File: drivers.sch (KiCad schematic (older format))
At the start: 40 parts, among them J10 Conn_01x04_Male, J11 Conn_01x04_Male, J12 Conn_01x02_Male, J13 Conn_01x02_Male, J14 Conn_01x02_Male, J15 Conn_01x02_Male, J4 Conn_01x04_Male, J5 Conn_01x04_Male, J6 Conn_01x02_Male, J7 Conn_01x02_Male, J8 Conn_01x02_Male, J9 Conn_01x02_Male

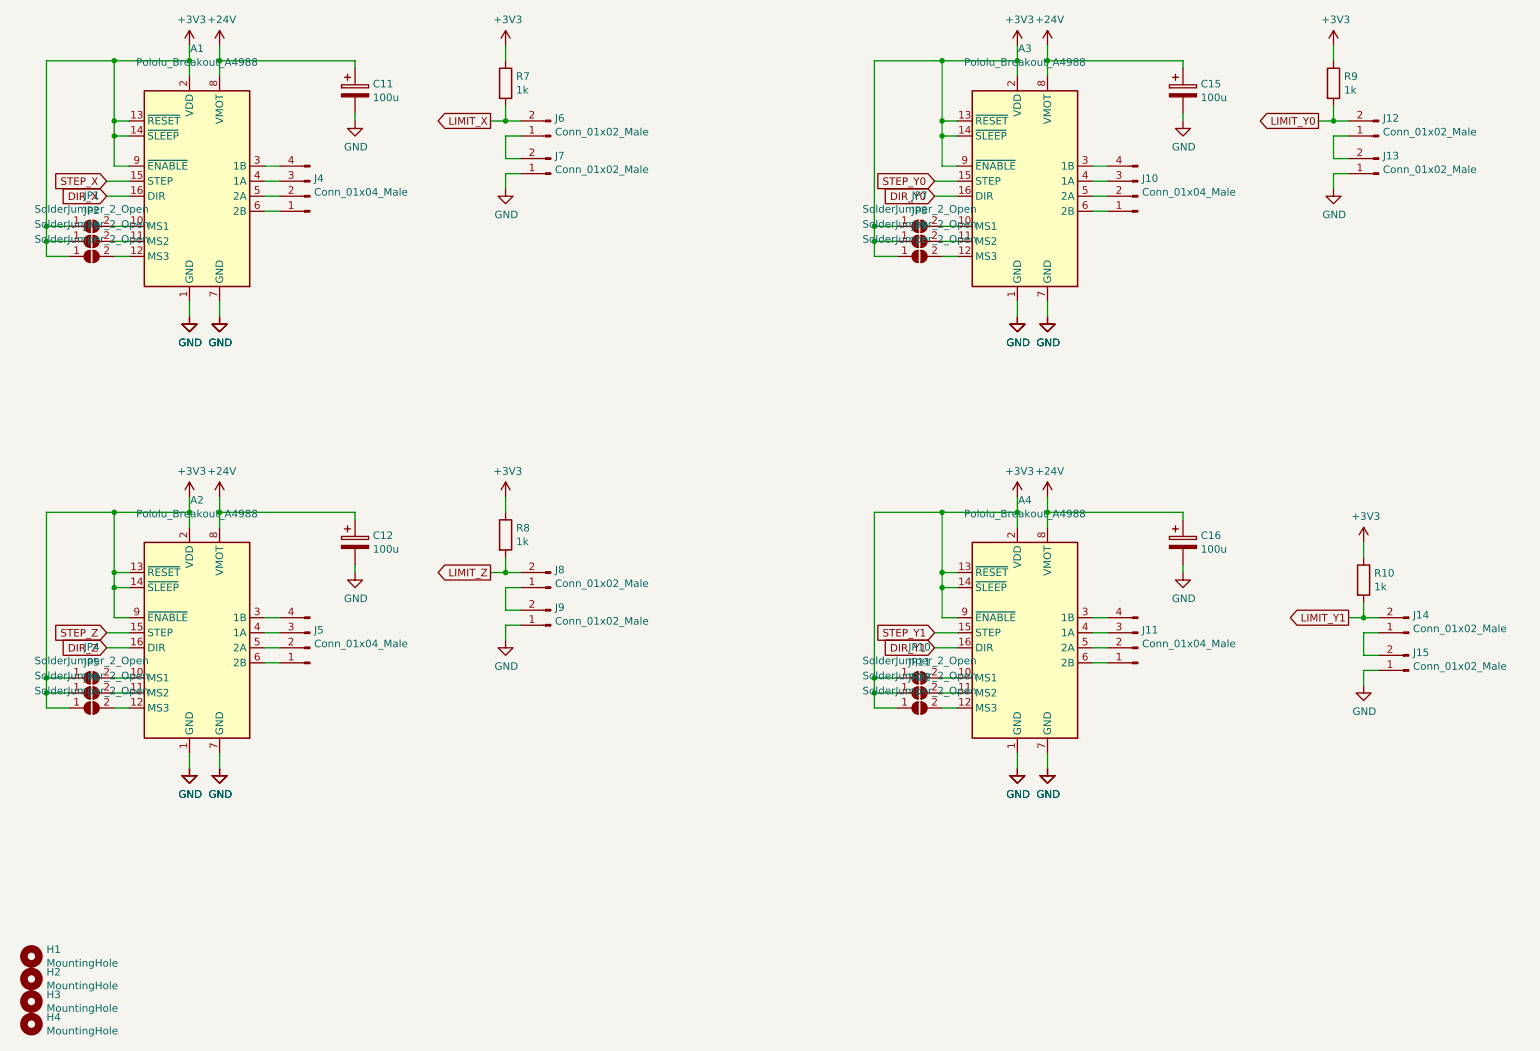
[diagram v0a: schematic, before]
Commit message: External drivers
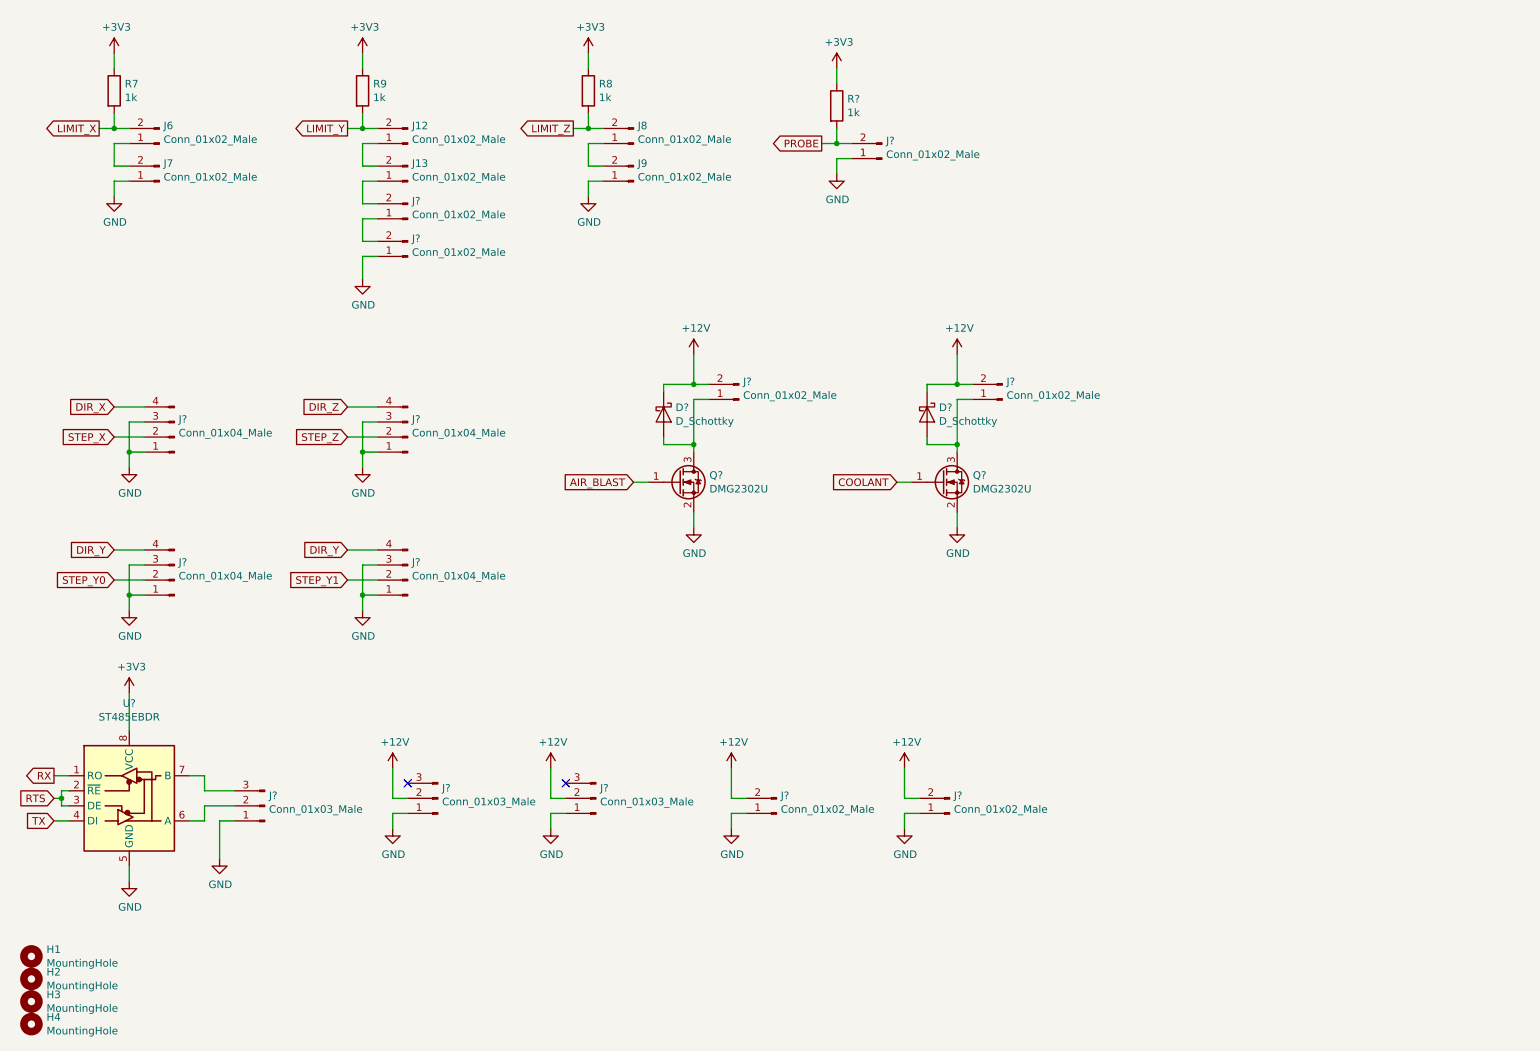
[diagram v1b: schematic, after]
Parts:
- removed A1, A2, A3, A4: Pololu_Breakout_A4988, Module:Pololu_Breakout-16_15.2x20.3mm, symbol Driver_Motor:Pololu_Breakout_A4988
- removed C11, C12, C15, C16: 100u, Capacitor_SMD:CP_Elec_8x10, symbol Device:CP
- removed J10, J11, J4, J5: Conn_01x04_Male, Connector_PinHeader_2.54mm:PinHeader_1x04_P2.54mm_Vertical, symbol Connector:Conn_01x04_Male
- removed J14, J15: Conn_01x02_Male, Connector_PinHeader_2.54mm:PinHeader_1x02_P2.54mm_Vertical, symbol Connector:Conn_01x02_Male
- removed JP1, JP10, JP11, JP12, JP2, JP3, JP4, JP5, JP6, JP7, JP8, JP9: SolderJumper_2_Open, Jumper:SolderJumper-2_P1.3mm_Open_Pad1.0x1.5mm, symbol Jumper:SolderJumper_2_Open
- removed R10: 1k, Resistor_SMD:R_1206_3216Metric_Pad1.42x1.75mm_HandSolder, symbol Device:R
- added D? (x2): D_Schottky, symbol Device:D_Schottky
- added J? (x7): Conn_01x02_Male, Connector_PinHeader_2.54mm:PinHeader_1x02_P2.54mm_Vertical, symbol Connector:Conn_01x02_Male
- added J? (x4): Conn_01x04_Male, symbol Connector:Conn_01x04_Male
- added J? (x3): Conn_01x03_Male, symbol Connector:Conn_01x03_Male
- added Q? (x2): DMG2302U, Package_TO_SOT_SMD:SOT-23, symbol Transistor_FET:DMG2302U
- added R?: 1k, Resistor_SMD:R_1206_3216Metric_Pad1.42x1.75mm_HandSolder, symbol Device:R
- added U?: ST485EBDR, Package_SO:SOIC-8_3.9x4.9mm_P1.27mm, symbol Interface_UART:ST485EBDR
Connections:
- net +3V3: now also R?.1, U?.8 (VCC)
- net DIR_X: now also J?.4 (Pin_4)
- net DIR_Z: now also J?.4 (Pin_4)
- net GND: now also J?.1 (Pin_1), J?.1 (Pin_1), J?.1 (Pin_1), J?.1 (Pin_1), J?.1 (Pin_1), J?.1 (Pin_1), J?.1 (Pin_1), J?.1 (Pin_1), J?.1 (Pin_1), J?.1 (Pin_1), J?.1 (Pin_1), J?.3 (Pin_3), J?.3 (Pin_3), J?.3 (Pin_3), J?.3 (Pin_3), Q?.2 (S), Q?.2 (S), U?.5 (GND); no longer J13.1 (Pin_1)
- net STEP_X: now also J?.2 (Pin_2)
- net STEP_Y0: now also J?.2 (Pin_2)
- net STEP_Y1: now also J?.2 (Pin_2)
- net STEP_Z: now also J?.2 (Pin_2)
- net LIMIT_Y0 renamed LIMIT_Y
- new net: J13.1 (Pin_1), J?.2 (Pin_2)
- new net: J?.1 (Pin_1), J?.2 (Pin_2)
- new net: J?.2 (Pin_2), U?.6 (A)
- new net: J?.3 (Pin_3), U?.7 (B)
- new net: D?.2 (A), J?.1 (Pin_1), Q?.3 (D) (x2)
- new net +12V: D?.1 (K), D?.1 (K), J?.2 (Pin_2), J?.2 (Pin_2), J?.2 (Pin_2), J?.2 (Pin_2), J?.2 (Pin_2), J?.2 (Pin_2)
- new net AIR_BLAST: Q?.1 (G)
- new net COOLANT: Q?.1 (G)
- new net DIR_Y: J?.4 (Pin_4), J?.4 (Pin_4)
- new net PROBE: J?.2 (Pin_2), R?.2
- new net RTS: U?.2 (~RE), U?.3 (DE)
- new net RX: U?.1 (RO)
- new net TX: U?.4 (DI)
- no-connect marks 0 -> 2
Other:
- moved on the sheet: J12, J13, J6, J7, J8, J9, R7, R8, R9
